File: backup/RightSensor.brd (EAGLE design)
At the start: 14.6 x 22.1 mm, 5 parts, among them X2 CNY70

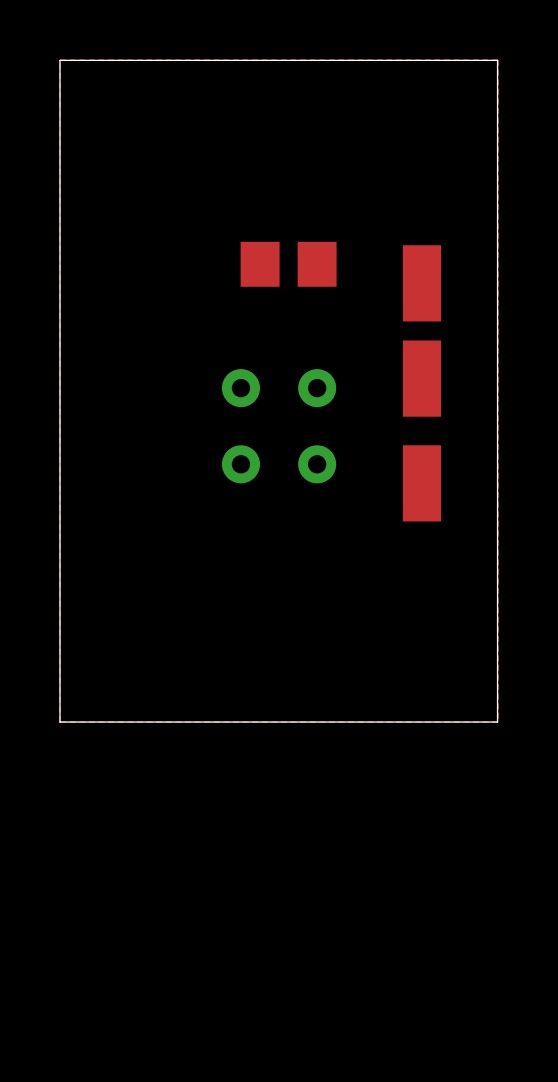
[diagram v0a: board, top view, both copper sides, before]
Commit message: Added code V1
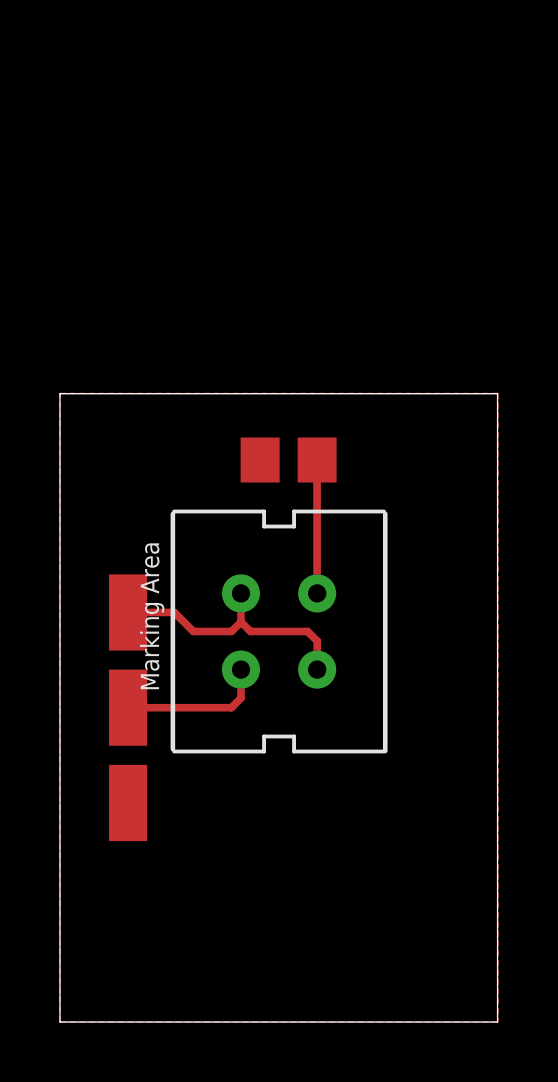
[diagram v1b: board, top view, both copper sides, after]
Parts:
- removed PAD4, PAD5, PAD6: WIREPADSMD1,27-254, wirepad:SMD1,27-2,54
- added PAD1, PAD2, PAD3: WIREPADSMD1,27-254, wirepad:SMD1,27-2,54
- moved X2 6.84 mm to (7.30, 13.0), flipped to the top, turned to 180 degrees
- moved R1 6.52 mm to (7.62, 18.7)
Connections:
- net GND: now also PAD3.1; no longer PAD6.1
- net SENSOR: now also PAD2.1; no longer PAD5.1
- net VCC: now also PAD1.1; no longer PAD4.1
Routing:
- net VCC: track 0.00 -> 8.87 mm
- net SENSOR: track 0.00 -> 4.85 mm
- net N$1: track 0.00 -> 4.45 mm
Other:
- board size 14.6 x 22.1 mm -> 14.6 x 20.9 mm
